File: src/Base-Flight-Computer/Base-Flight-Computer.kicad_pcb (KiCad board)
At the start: 4 copper layers, 41 x 20.3 mm, 58 parts, among them J1 Jumper_NO, P1 1984659, P2 USB, P3 0530470610, P4 1984659, P5 B2B-PH-K-SLFSN_JST, Q1 QS5U17TR, Q2 2N7002W-7-F, Q3 2N7002W-7-F, Q4 QS5U17TR, Q5 2N7002W-7-F, Q6 2N7002W-7-F, U1 STM32G4A1KEU6, U2 BMP390, U3 LMS8117AMP-3.3_NOPB, U4 SST25VF040B-50-4I-S2AE-T, Y1 ECS-240-18-33-JGN-TR

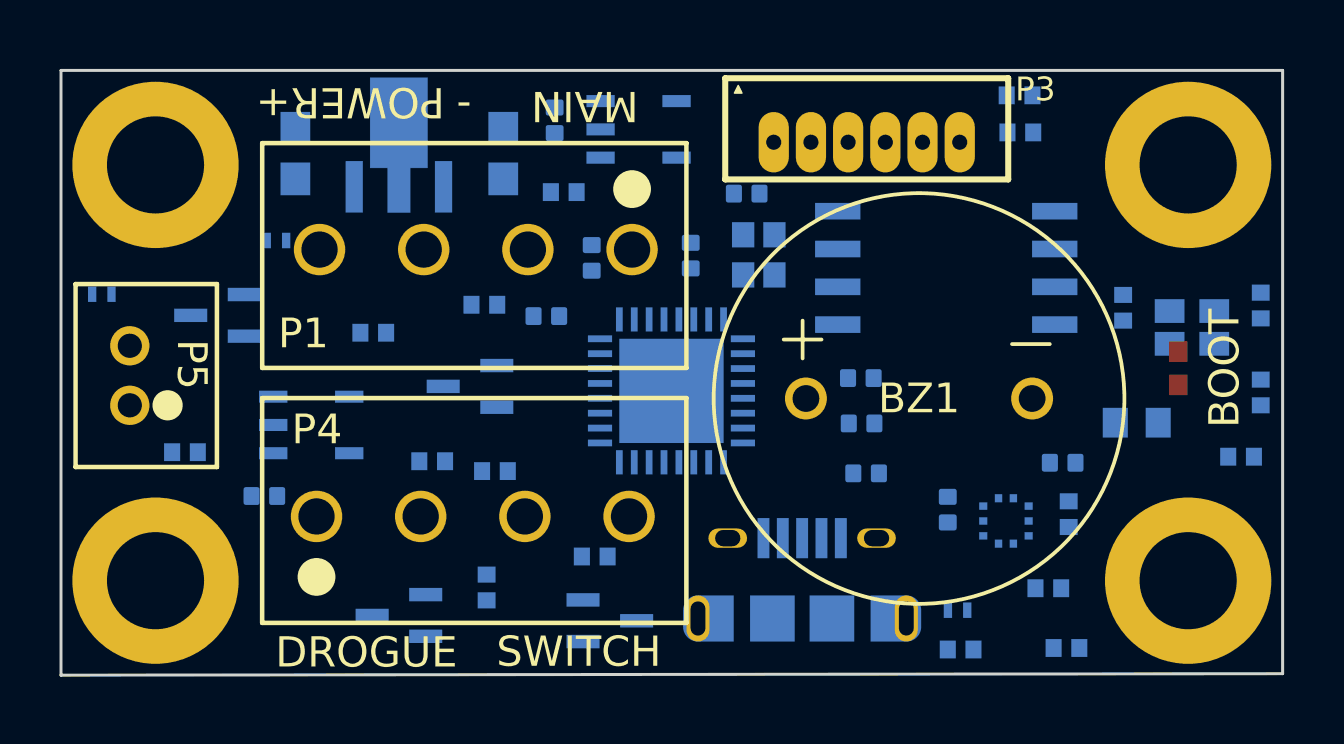
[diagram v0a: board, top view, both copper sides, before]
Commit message: created new project for preliminary hardware testing
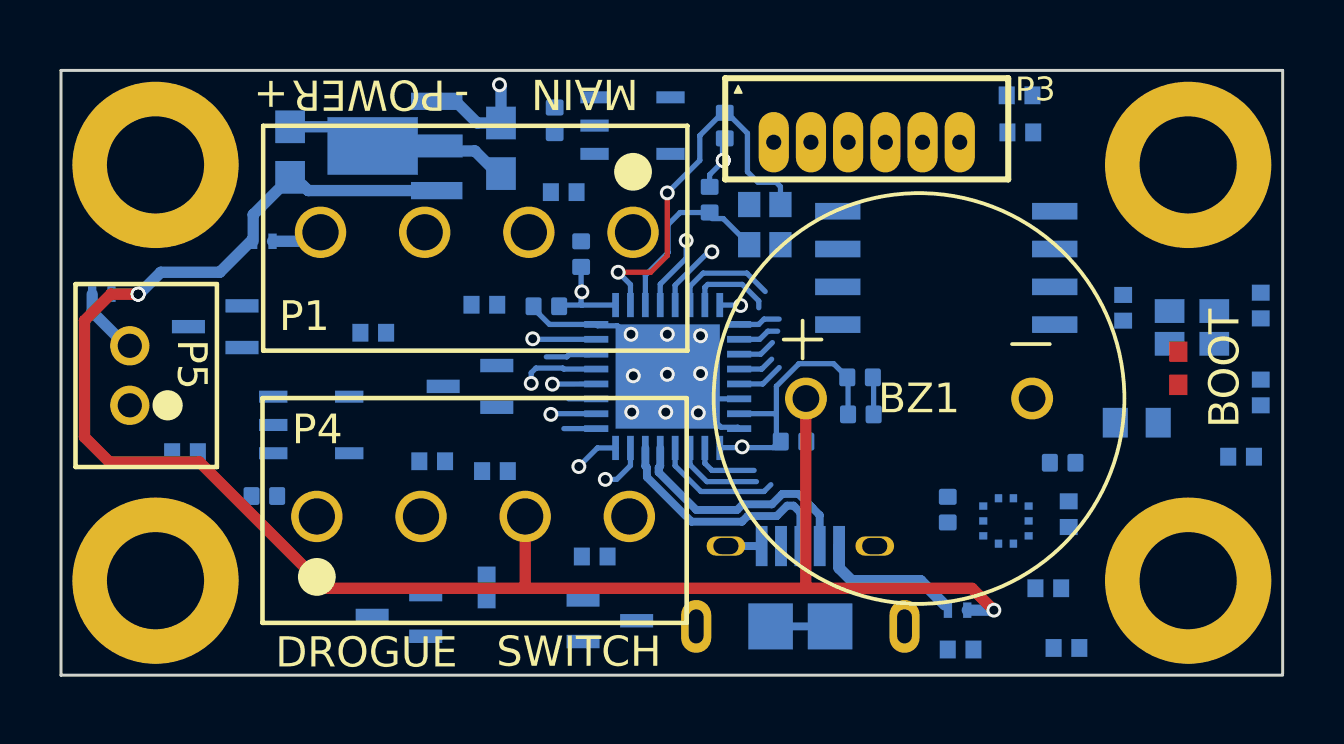
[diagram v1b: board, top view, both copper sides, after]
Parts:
- moved C10 4.52 mm to (149.3, 83.1), turned to -90 degrees
- moved C1 2.37 mm to (151.6, 93.8)
- moved C4 1.99 mm to (153.9, 92.8)
- moved C11 1.26 mm to (148.8, 85.6), turned to 90 degrees
- moved Y1 1.04 mm to (150.6, 86.5), turned to -90 degrees
- moved P1 0.58 mm to (146.2, 86.7)
- moved U1 0.50 mm to (147.4, 91.6)
- moved D4 0.46 mm to (133.8, 87.0)
- moved U3 0.45 mm to (138.0, 83.8), turned to 180 degrees
- moved Q2 0.39 mm to (132.2, 89.9)
- moved C2 0.38 mm to (144.5, 87.5)
- moved C3 0.33 mm to (143.3, 89.2)
- moved P2 0.27 mm to (151.8, 100.0)
- moved Q1 0.24 mm to (146.2, 83.1)
- moved C13 0.19 mm to (141.8, 83.9), turned to -90 degrees
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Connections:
- U1 pad 30: STATUS_B -> ~{MAIN_CONT}
- U1 pad 33: unconnected-(U1-Exposed_Pad-Pad33) -> Earth
- U1 pad 9: ~{MAIN_CONT} -> STATUS_B
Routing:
- net VIN: track 0.00 -> 61.0 mm, vias 0 -> 3
- net Earth: track 0.00 -> 18.0 mm, vias 0 -> 11
- net 3.3V: track 0.00 -> 15.5 mm, vias 0 -> 3
- net OSC_IN: track 0.00 -> 12.8 mm, vias 0 -> 2
- net USB_D-: track 0.00 -> 8.48 mm
- net USB_D+: track 0.00 -> 8.22 mm
- net OSC_OUT: track 0.00 -> 6.03 mm
- net 5V: track 0.00 -> 4.80 mm
- net USB_DETECT: track 0.00 -> 4.27 mm
- net ~{SWITCH}: track 0.00 -> 3.60 mm
- net BP_SCL: track 0.00 -> 3.03 mm
- net BEEP: track 0.00 -> 2.91 mm
- net STATUS_G: track 0.00 -> 2.75 mm, vias 0 -> 1
- net NRST: track 0.00 -> 2.53 mm, vias 0 -> 1
- net VBAT_SENSE: track 0.00 -> 2.37 mm, vias 0 -> 1
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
